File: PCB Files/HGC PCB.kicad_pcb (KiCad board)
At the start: 2 copper layers, 174.5 x 69.9 mm, 151 parts, among them J1 MPU6050, J10 Conn_01x07_Pin, J11 Conn_01x07_Pin, J12 Conn_01x04_Pin, J13 Conn_01x07_Pin, J14 USB_C_Receptacle_USB2.0_16P, J15 Conn_01x08_Pin, J16 Conn_01x08_Pin, J17 B2B-XH-A__LF__SN_, J18 B2B-XH-A__LF__SN_, J2 DISPLAY, J3 SDCARD, J4 Conn_01x07_Pin, J5 Conn_01x07_Pin, J6 Conn_01x07_Pin, J7 Conn_01x05_Pin, J8 Conn_01x05_Pin, J9 Conn_01x07_Pin, SW1 SW_SPDT, SW2 SW_Push, SW3 SW_Push, SW4 SW_Push, SW5 SW_Push, SW6 SW_Push, SW7 SW_Push, SW8 SW_Push, U1 STM32F407VGTx, U2 JOYSTICK, U3 AMS1117-3.3, U4 CP2102N-Axx-xQFN28, U5 MP1584EN-LF, Y1 Crystal_GND24

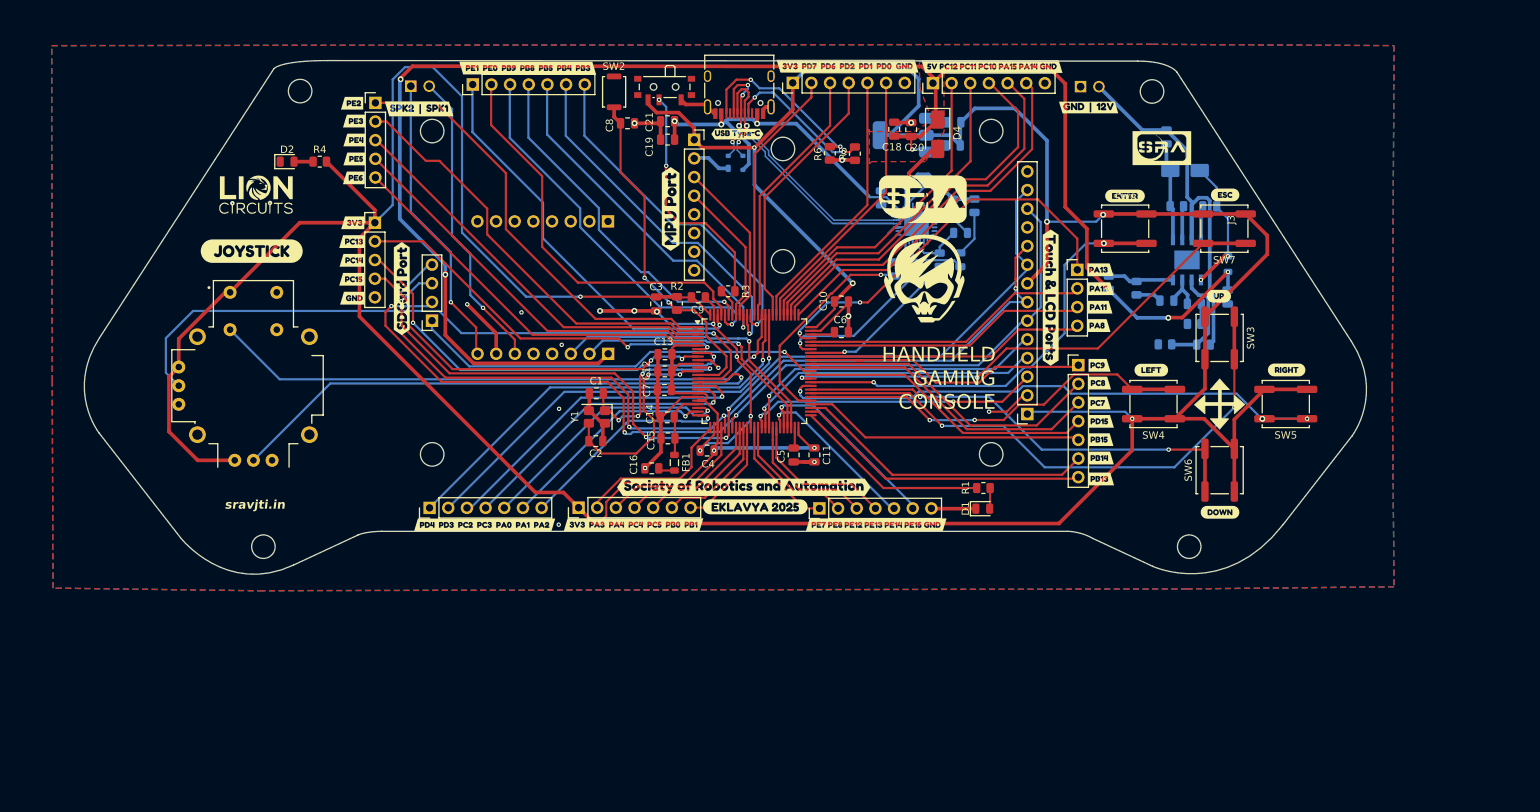
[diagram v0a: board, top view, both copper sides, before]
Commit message: Add files via upload
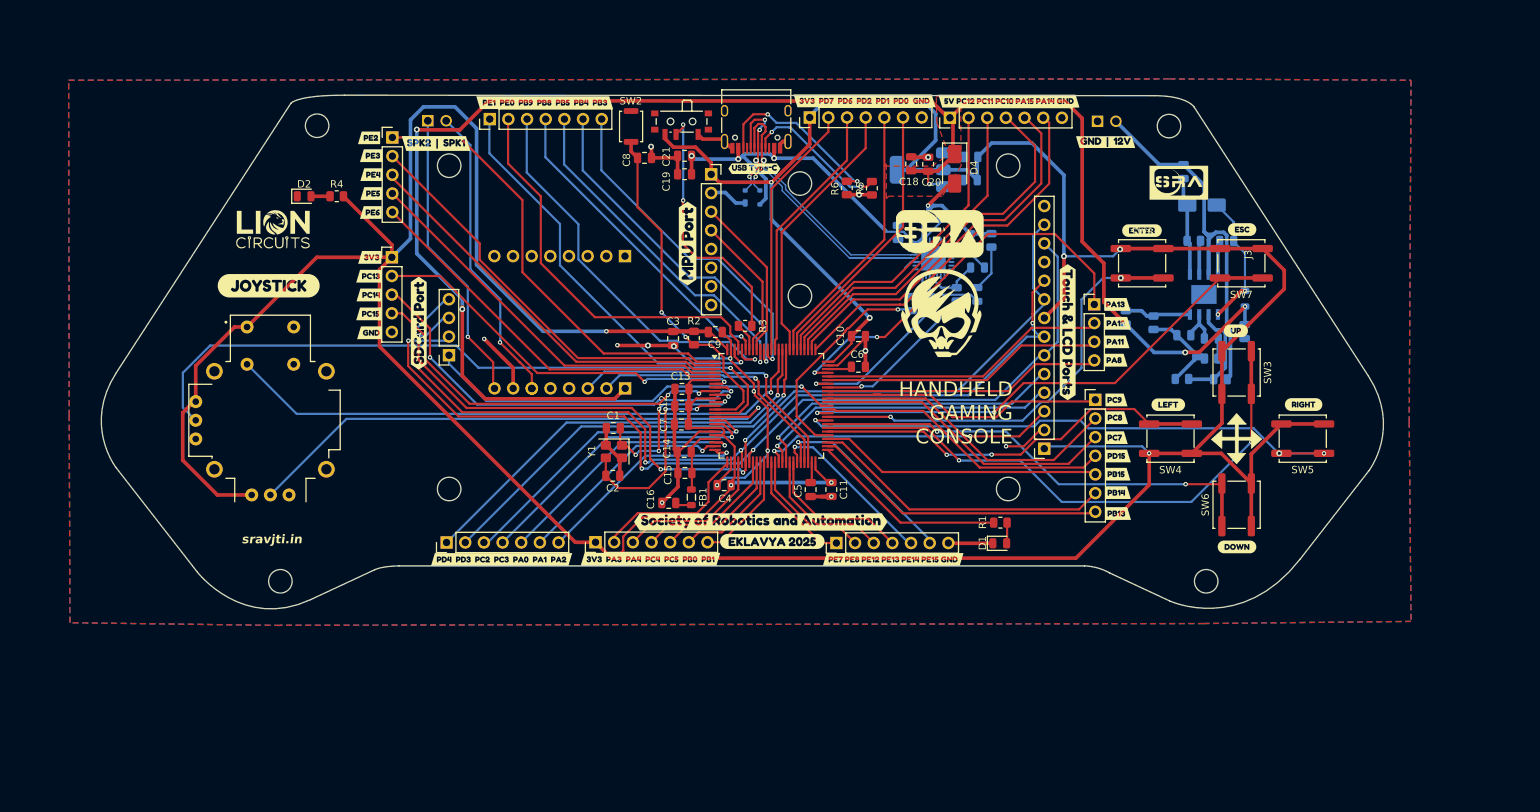
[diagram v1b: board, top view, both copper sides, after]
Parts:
- removed the G*** at (170.6, 90.0)
- removed the G*** at (170.4, 79.2)
- removed the G*** at (135.4, 107.8)
- removed the G*** at (149.1, 97.6)
- removed kibuzzard-68C938FF: G***, kibuzzard-68C938FF
- added ?: , , F.Cu at (117.2, 105.0)
- added G***: LOGO, logos:sra_skull_big, F.Cu at (172.9, 94.7)
- added G***: LOGO, Logos:sra_logo_big, F.Cu at (172.7, 83.9)
- added G***: LOGO, logos:sra_skull_big, B.Cu at (151.4, 102.3)
- added G***: LOGO, Logos:sra_logo_big, B.Cu at (137.7, 112.5)
- added kibuzzard-68D3B1B5: G***, kibuzzard-68D3B1B5, B.Cu at (119.7, 83.3)
- moved J16 5.26 mm to (129.8, 87.0)
- moved C10 5.25 mm to (161.6, 97.8)
- moved C16 5.25 mm to (135.8, 120.5)
- moved C25 5.25 mm to (167.0, 83.7)
- moved C29 5.25 mm to (214.2, 97.2)
- moved C4 5.25 mm to (143.3, 118.1)
- moved C6 5.25 mm to (161.6, 102.0)
- moved C7 5.25 mm to (137.5, 109.9)
- moved C9 5.25 mm to (142.1, 97.3)
- moved D1 5.25 mm to (180.8, 126.0)
- moved D3 5.25 mm to (147.2, 79.0)
- moved G*** 5.25 mm to (81.9, 83.3)
- moved H8 5.25 mm to (87.9, 69.2)
- moved J2 5.25 mm to (186.9, 113.2)
- moved J6 5.25 mm to (174.1, 68.1)
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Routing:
- net /3.3V: track 621.1 -> 637.4 mm
- net GND: track 165.9 -> 178.3 mm, vias 22 -> 16
- net /VBUS: track 72.1 -> 75.6 mm
- net /PB8: track 46.5 -> 43.5 mm
- net /sw_boot0: track 32.4 -> 35.1 mm
- net /PB4: track 49.0 -> 46.6 mm
- net /12V: track 55.9 -> 57.7 mm
- net /HSE_OUT: track 29.3 -> 27.7 mm
- net /PB9: track 52.8 -> 54.1 mm
- net /PE2: track 61.0 -> 62.3 mm
- net /5V: track 226.4 -> 225.2 mm
- net /PC2: track 45.2 -> 44.3 mm
- net /PB3: track 46.7 -> 45.8 mm
- net /DC: track 42.7 -> 43.6 mm
- net /Push3: track 80.0 -> 79.2 mm
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
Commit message: Add files via upload
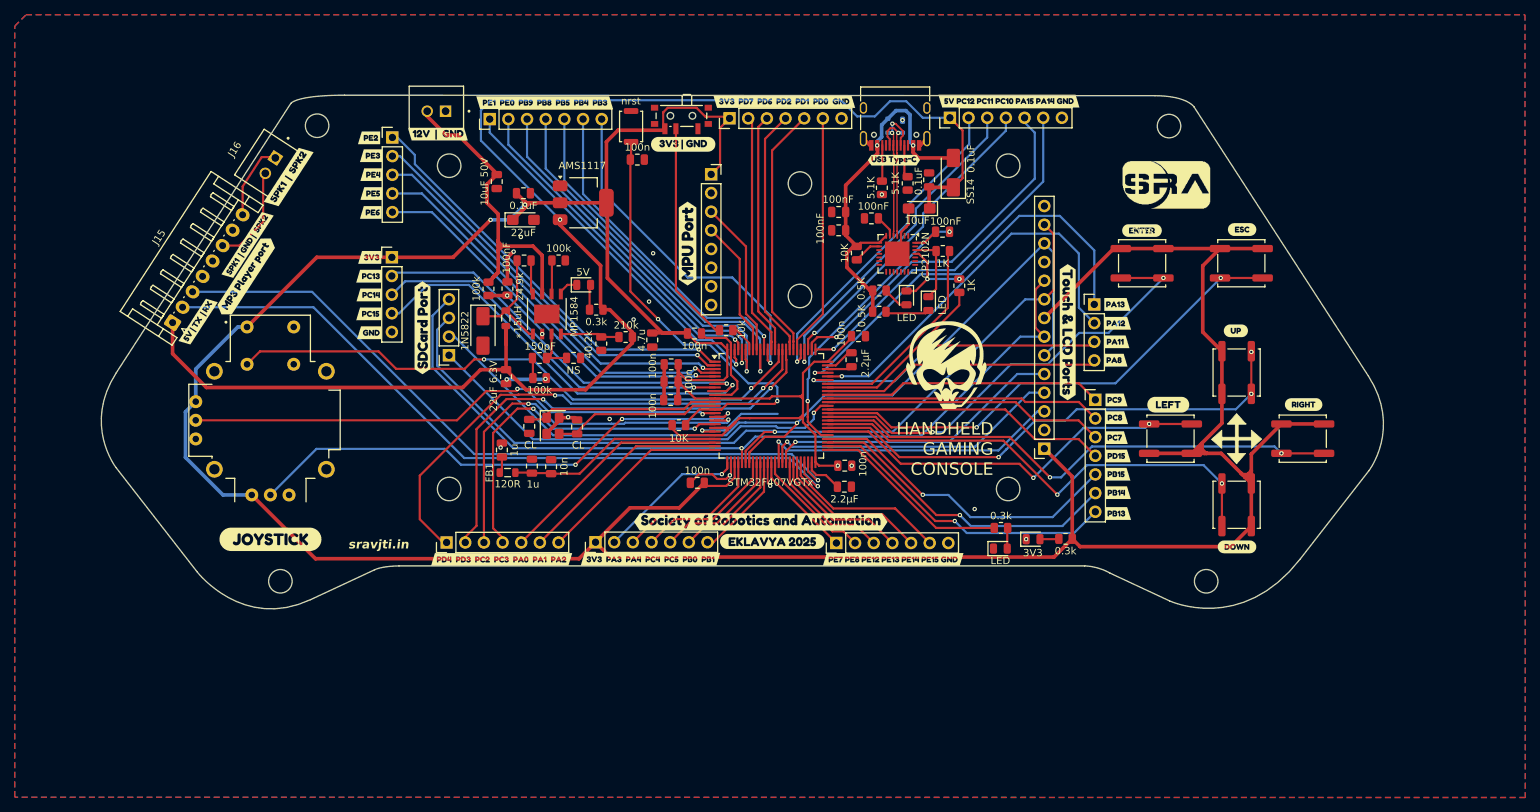
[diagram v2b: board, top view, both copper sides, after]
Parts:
- removed ?: , 
- removed the G*** at (205.2, 77.0)
- removed J18: B2B-XH-A__LF__SN_, JST:JST_B2B-XH-A__LF__SN_
- removed the REF** at (222.4, 120.2)
- removed the REF** at (165.2, 111.5)
- removed kibuzzard-68C923F6: G***, kibuzzard-68C923F6
- removed kibuzzard-68C931ED: G***, kibuzzard-68C931ED
- removed kibuzzard-68C939EA: G***, kibuzzard-68C939EA
- removed kibuzzard-68C93B18: G***, kibuzzard-68C93B18
- added D8: 5V, LED_SMD:LED_0805_2012Metric, F.Cu at (124.2, 90.9)
- added R18: 0.3k, Resistor_SMD:R_0805_2012Metric, F.Cu at (125.9, 94.2)
- added REF**: KiCad-Logo2_6mm_SilkScreen, symbols1:KiCad-Logo2_6mm_SilkScreen, B.Cu at (213.2, 111.2)
- added REF**: OSHW-Logo2_7.3x6mm_SilkScreen, Symbol:OSHW-Logo2_7.3x6mm_SilkScreen, B.Cu at (221.4, 120.6)
- added kibuzzard-6946C392: G***, kibuzzard-6946C392, F.Cu at (104.4, 70.4)
- added kibuzzard-6946C401: G***, kibuzzard-6946C401, F.Cu at (84.1, 76.2)
- added kibuzzard-6946C61F: G***, kibuzzard-6946C61F, F.Cu at (137.8, 71.7)
- added kibuzzard-694FD5EF: G***, kibuzzard-694FD5EF, F.Cu at (71.7, 95.9)
- added kibuzzard-694FDB00: G***, kibuzzard-694FDB00, F.Cu at (203.8, 107.2)
- C17, C22, C24, C25, C26, C27, C28, C29, D5, D6, D7, J17, L1, R10, R11, R12, R13, R14, R15, R16, R17, R7, R8, R9, kibuzzard-68C93B2B, kibuzzard-68D3B1B5: moved to F.Cu
- C18: footprint Capacitor_SMD:C_0805_2012Metric -> Capacitor_Tantalum_SMD:CP_EIA-3216-10_Kemet-I_HandSolder
- C23: footprint Capacitor_SMD:C_0805_2012Metric -> Capacitor_Tantalum_SMD:CP_EIA-3216-10_Kemet-I_HandSolder; moved to F.Cu
- C5, C6: value 2.2 µF -> 2.2µF
- G***: moved to B.Cu
- J15: footprint Connector_PinSocket_2.54mm:PinSocket_1x08_P2.54mm_Vertical -> Connector_JST:JST_EH_S8B-EH_1x08_P2.50mm_Horizontal; moved to F.Cu
- J16: value Conn_01x08_Pin -> B2B-XH-A__LF__SN_; footprint Connector_PinSocket_2.54mm:PinSocket_1x08_P2.54mm_Vertical -> JST:JST_B2B-XH-A__LF__SN_; moved to F.Cu
- U3: value AMS1117-3.3 -> AMS1117; moved to F.Cu
- U4: value CP2102N-Axx-xQFN28 -> CP2102N; moved to F.Cu
- U5: value MP1584EN-LF -> MP1584; moved to F.Cu
- moved D2 109.6 mm to (185.4, 125.5)
- moved R4 109.6 mm to (189.8, 125.4)
- moved C29 100.7 mm to (113.6, 103.3)
- moved L1 100.6 mm to (113.6, 95.4)
- moved R9 100.4 mm to (111.2, 91.4), turned to -90 degrees
- moved D5 99.3 mm to (110.5, 97.1), turned to -90 degrees
- moved C22 95.7 mm to (116.1, 87.5), turned to 0 degrees
- moved C17 93.5 mm to (112.4, 76.8)
- moved R10 92.6 mm to (113.8, 91.4), turned to 90 degrees
- moved C26 91.5 mm to (118.2, 100.8), turned to 180 degrees
- moved R12 91.4 mm to (118.2, 103.5), turned to 0 degrees
- moved U5 89.5 mm to (119.2, 94.8)
- moved R7 86.5 mm to (120.8, 87.5), turned to 180 degrees
- moved G*** 84.7 mm to (161.8, 111.6), turned to 180 degrees
- moved C27 83.1 mm to (122.8, 100.8), turned to 0 degrees
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- renumbered SW2 to nrst
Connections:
- J16 pad 1: unconnected-(J16-Busy-Pad1) -> /SPK2
- J16 pad 2: unconnected-(J16-USB--Pad2) -> /SPK1
- J17 pad 1: /SPK2 -> GND
- J17 pad 2: /SPK1 -> /12V
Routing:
- net GND: track 178.3 -> 77.6 mm, vias 16 -> 18
- net /3.3V: track 637.4 -> 542.5 mm, vias 8 -> 3
- net /USART3_TX: track 35.4 -> 100.7 mm
- net /USART3_RX: track 39.6 -> 99.4 mm
- net /D+: track 54.0 -> 18.1 mm, vias 4 -> 1
- net /SPK2: track 40.2 -> 10.5 mm, vias 1 -> 0
- net /SPK1: track 41.3 -> 13.9 mm, vias 1 -> 0
- net /D-: track 42.6 -> 19.3 mm
- net /V: track 95.9 -> 74.1 mm, vias 1 -> 2
- net /VBUS: track 75.6 -> 53.9 mm, vias 4 -> 2
- net Net-(U1-VDDA): track 9.42 -> 29.2 mm
- net Net-(J14-CC2): track 24.5 -> 4.89 mm, vias 2 -> 0
- net /5V: track 225.2 -> 206.8 mm, vias 6 -> 1
- net Net-(J14-CC1): track 20.1 -> 4.45 mm, vias 2 -> 0
- net /NRST: track 47.6 -> 62.1 mm
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- removed copper zone on F.Cu, net /5V
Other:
- board text added: "0.1uF"
- board text added: "3V3"
- board text added: "BY, MUSTAFA T R ASHISH NERLEKAR PAARTH SHIRSAT"
- board text removed: "BY, MUSTAFA T R ASHISH NERLEKAR PAARTH SHIRSAT AND MENTORS, VISHAL MUTHA PIYUSH PATLE SHAURYA RANE"
- board text removed: "R8"
